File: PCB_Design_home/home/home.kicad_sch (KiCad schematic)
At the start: 54 parts, among them J1 USB_C_Receptacle_USB2.0_16P, J2 Conn_01x05_Socket, Q1 2N3904, Q2 2N3904, SW1 SW_Push, SW2 SW_Push, SW3 SW_Push, SW4 SW_Push, U1 ESP32-C3-WROOM-02, U2 CP2102N-Axx-xQFN28, U3 ULN2003A, U4 BME680, U5 AMS1117-3.3

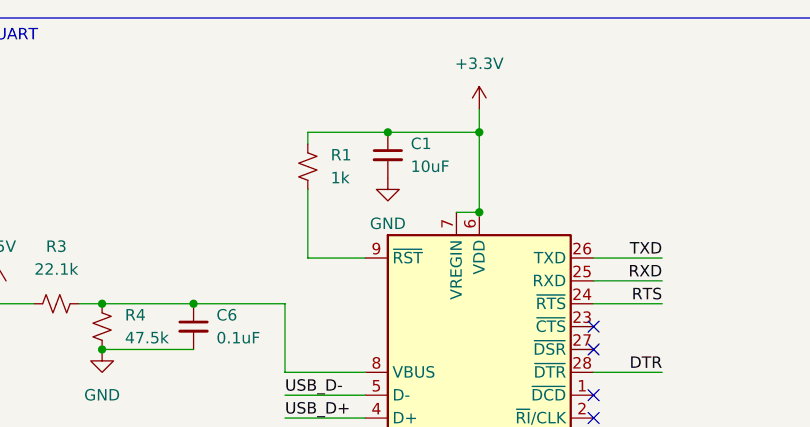
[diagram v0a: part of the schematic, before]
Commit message: Update
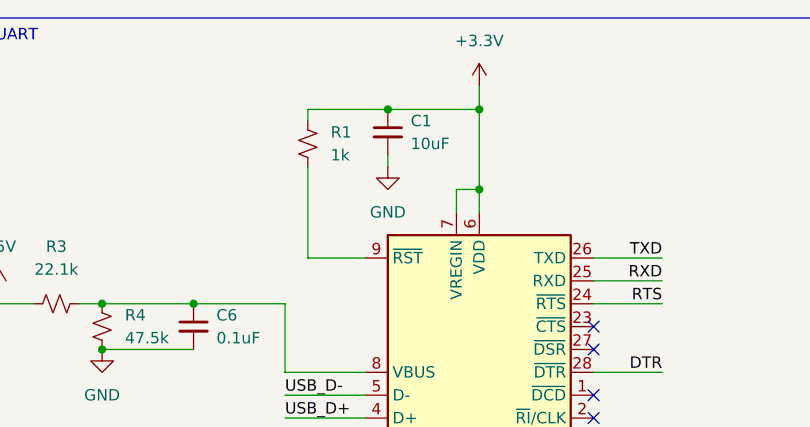
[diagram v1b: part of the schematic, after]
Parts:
- removed CR1, CR2, CR3: GG0402052R542P, Home_Sensor_foot_lib:TVS_GG0402_KAV, symbol Hone_Sensor_symbol_lib:GG0402052R542P
- added CR1, CR2, CR3: GG0402052R542P, Home_Sensor_foot_lib:TVS_GG0402_KAV, symbol Home_Sensor_Symbol_lib:GG0402052R542P
- C1, C10, C11, C12, C13, C14, C15, C16, C17, C2, C3, C4, C5, C6, C7, C8, C9: footprint (none) -> Capacitor_SMD:C_0603_1608Metric_Pad1.08x0.95mm_HandSolder
- D1, D2, D3, D4, D5: footprint (none) -> LED_SMD:LED_0603_1608Metric_Pad1.05x0.95mm_HandSolder
- J2: footprint (none) -> Connector_PinSocket_2.54mm:PinSocket_1x05_P2.54mm_Vertical
- R1, R10, R11, R12, R13, R14, R15, R16, R2, R3, R4, R5, R6, R7, R8, R9: footprint (none) -> Resistor_SMD:R_0603_1608Metric_Pad0.98x0.95mm_HandSolder
- SW1, SW2, SW3, SW4: footprint (none) -> Home_Sensor_foot_lib:SW4_1825910-B_TEC
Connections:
- net +5V: now also CR3.1
- net GND: now also CR1.2, CR2.2, CR3.2
- net USB_D+: now also CR1.1
- net USB_D-: now also CR2.1
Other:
- moved on the sheet: C1, R1
